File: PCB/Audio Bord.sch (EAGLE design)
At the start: 51 parts, among them J1 Audio, P4SMAJ16A TVS-16V, T1 IRFB4229, U1 CD74HC14EN14, U2 NE555DRD8, U3 UCC27524DRD0008A_L

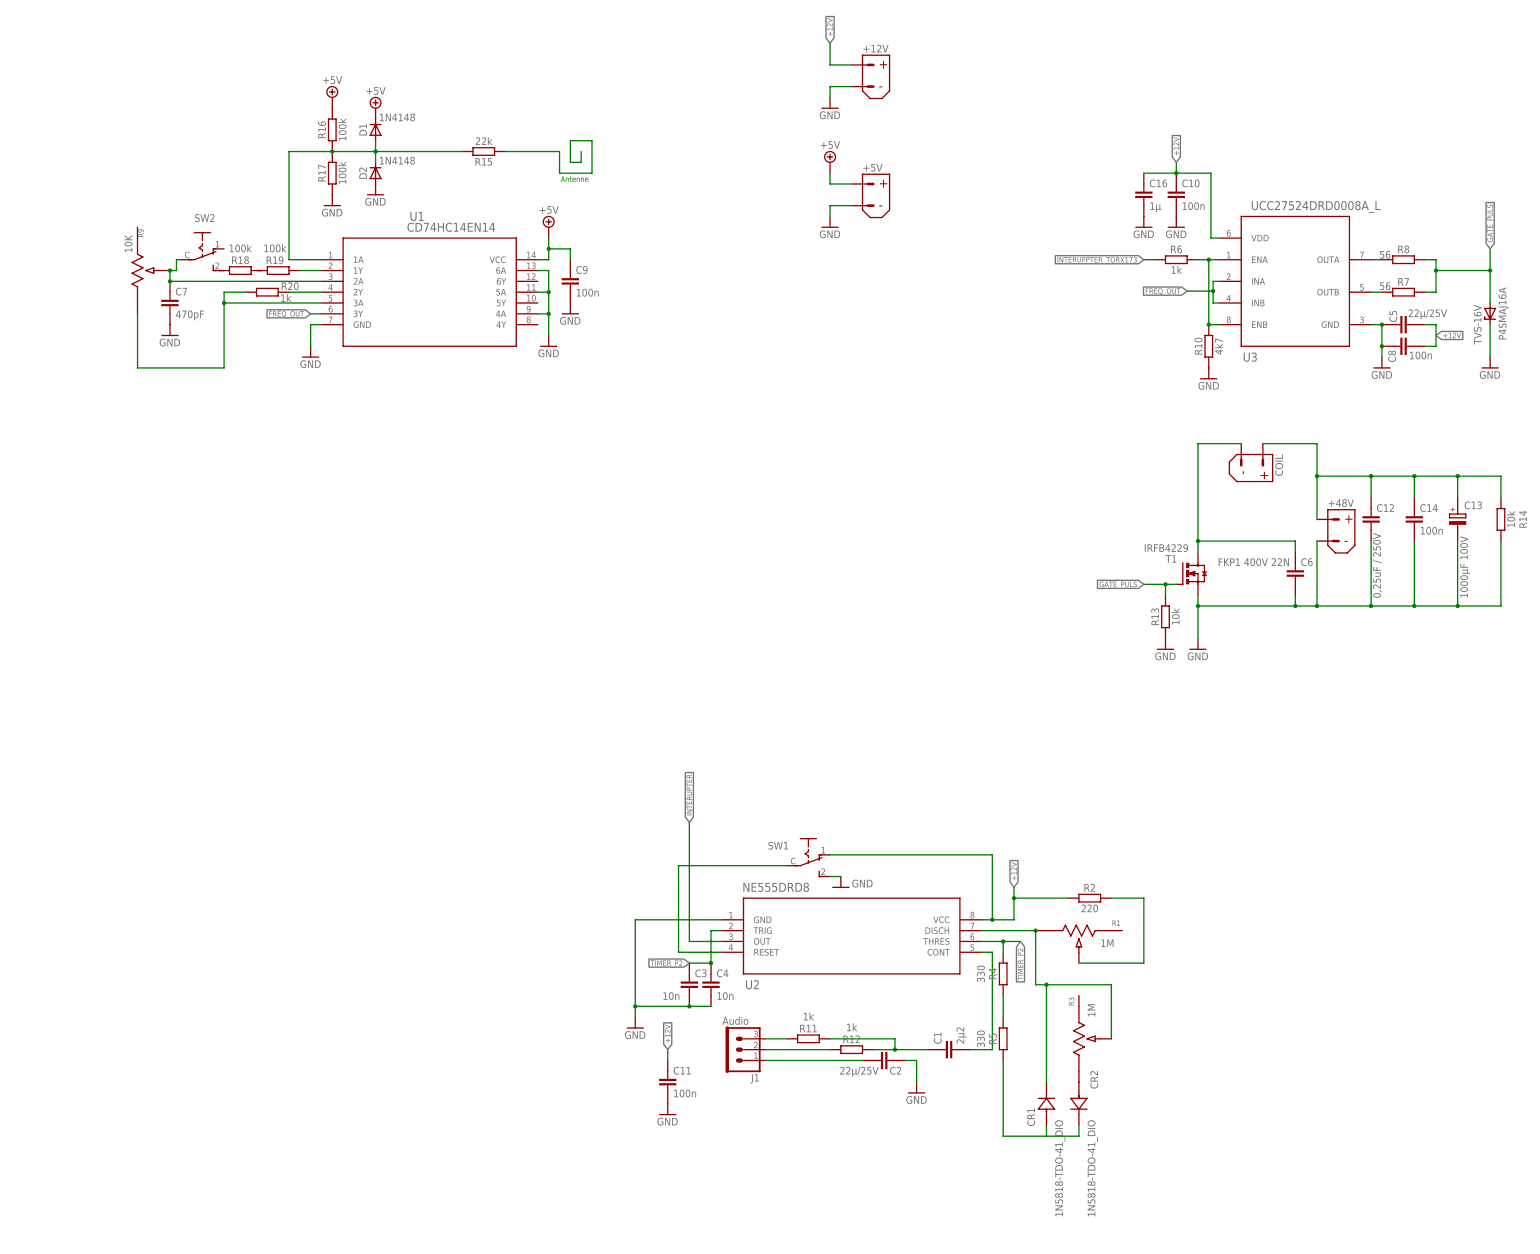
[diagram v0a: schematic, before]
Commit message: audio interupter
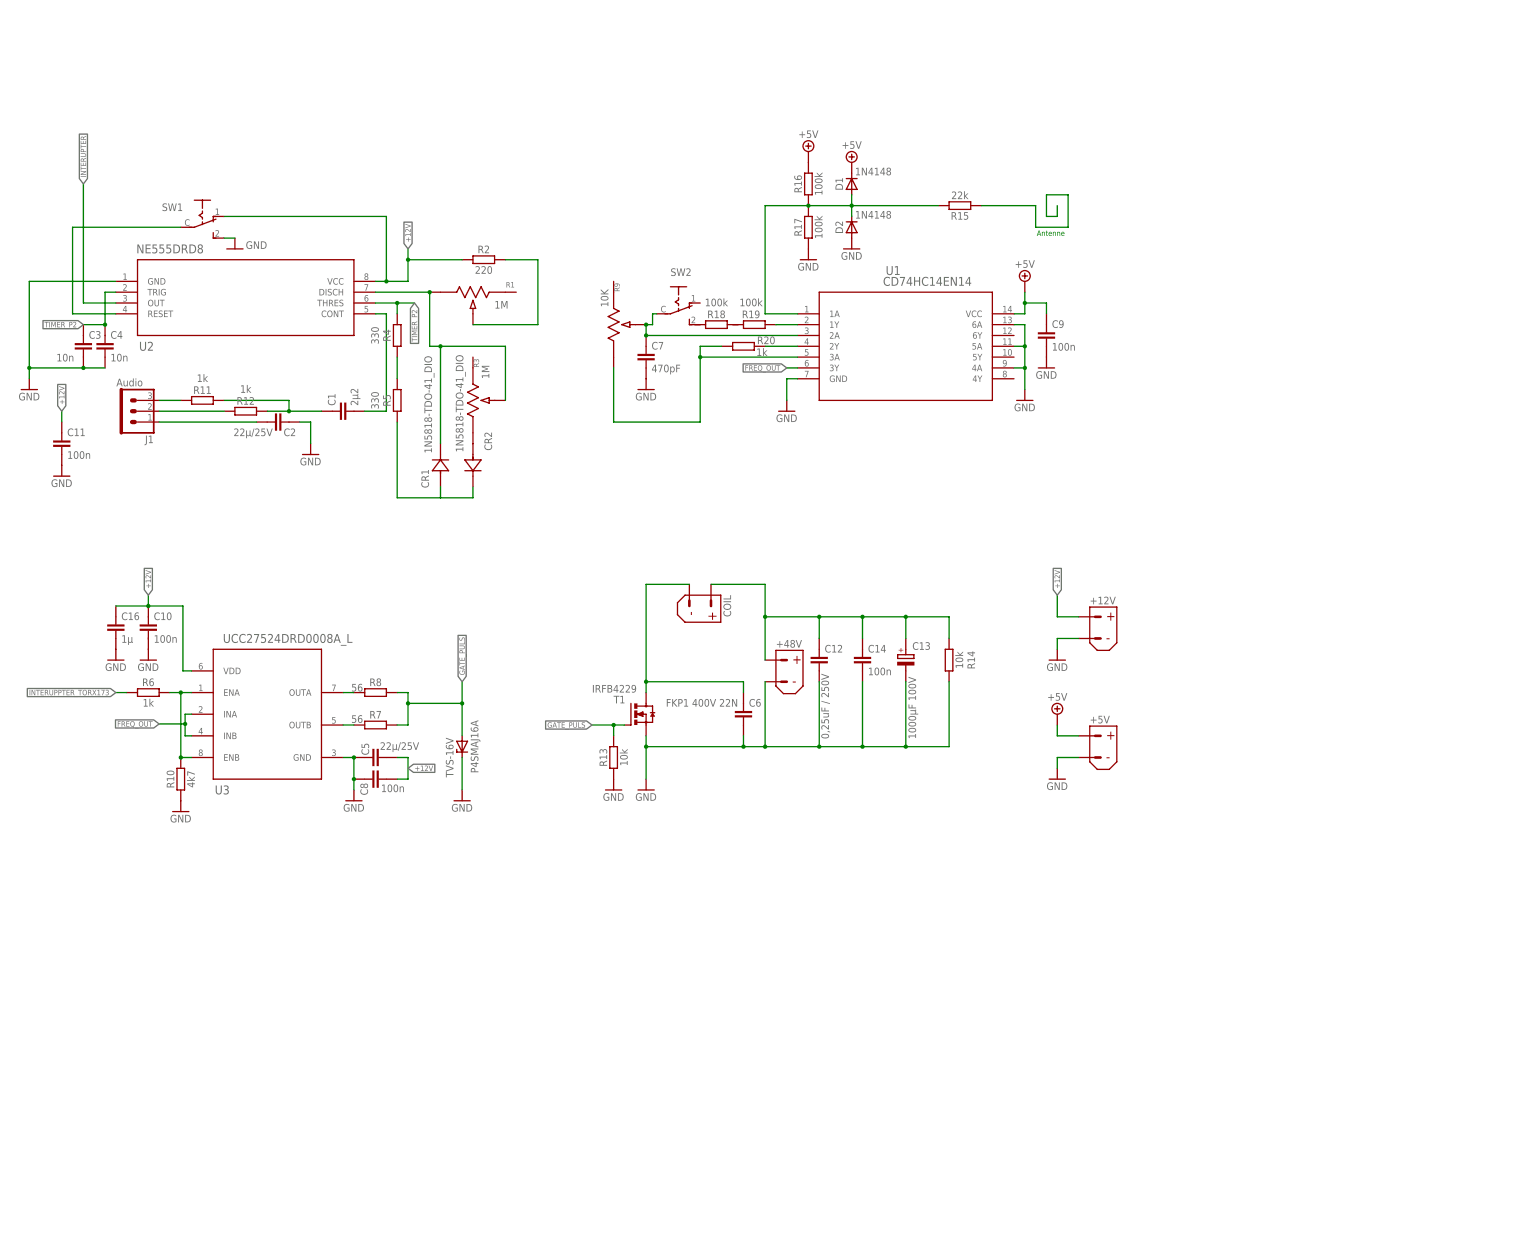
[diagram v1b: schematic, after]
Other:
- moved on the sheet: +12V, +48V, +5V, C1, C10, C11, C12, C13, C14, C16, C2, C3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
